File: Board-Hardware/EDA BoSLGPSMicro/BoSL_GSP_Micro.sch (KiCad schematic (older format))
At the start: 45 parts, among them CON1 Micro_SD_Card, CON2 BARREL_JACK, IC1 ATMEGA328-P, IC2 SIM7000, J7 USB_B_Micro, P2 CONN_01X04, P4 CONN_01X04, P7 CONN_01X04, SW1 SPST, U1 MCP1700T-3302E/TT, U3 MSQA6V1W5T2G, U4 74HC126, U5 FT232RL, Y1 8 MHz

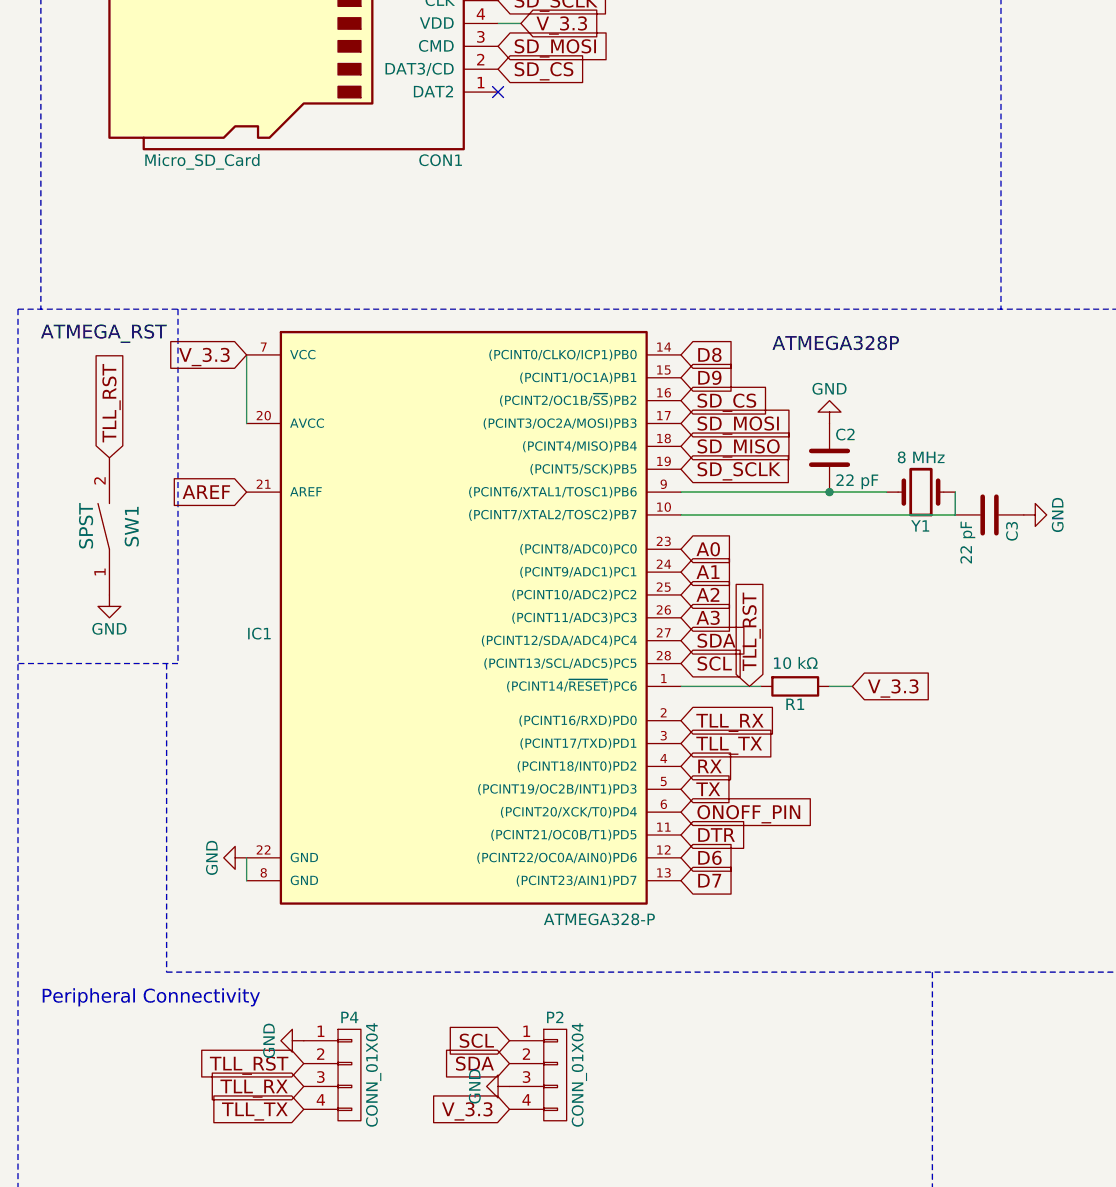
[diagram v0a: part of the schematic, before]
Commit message: layout progress of gps micro board
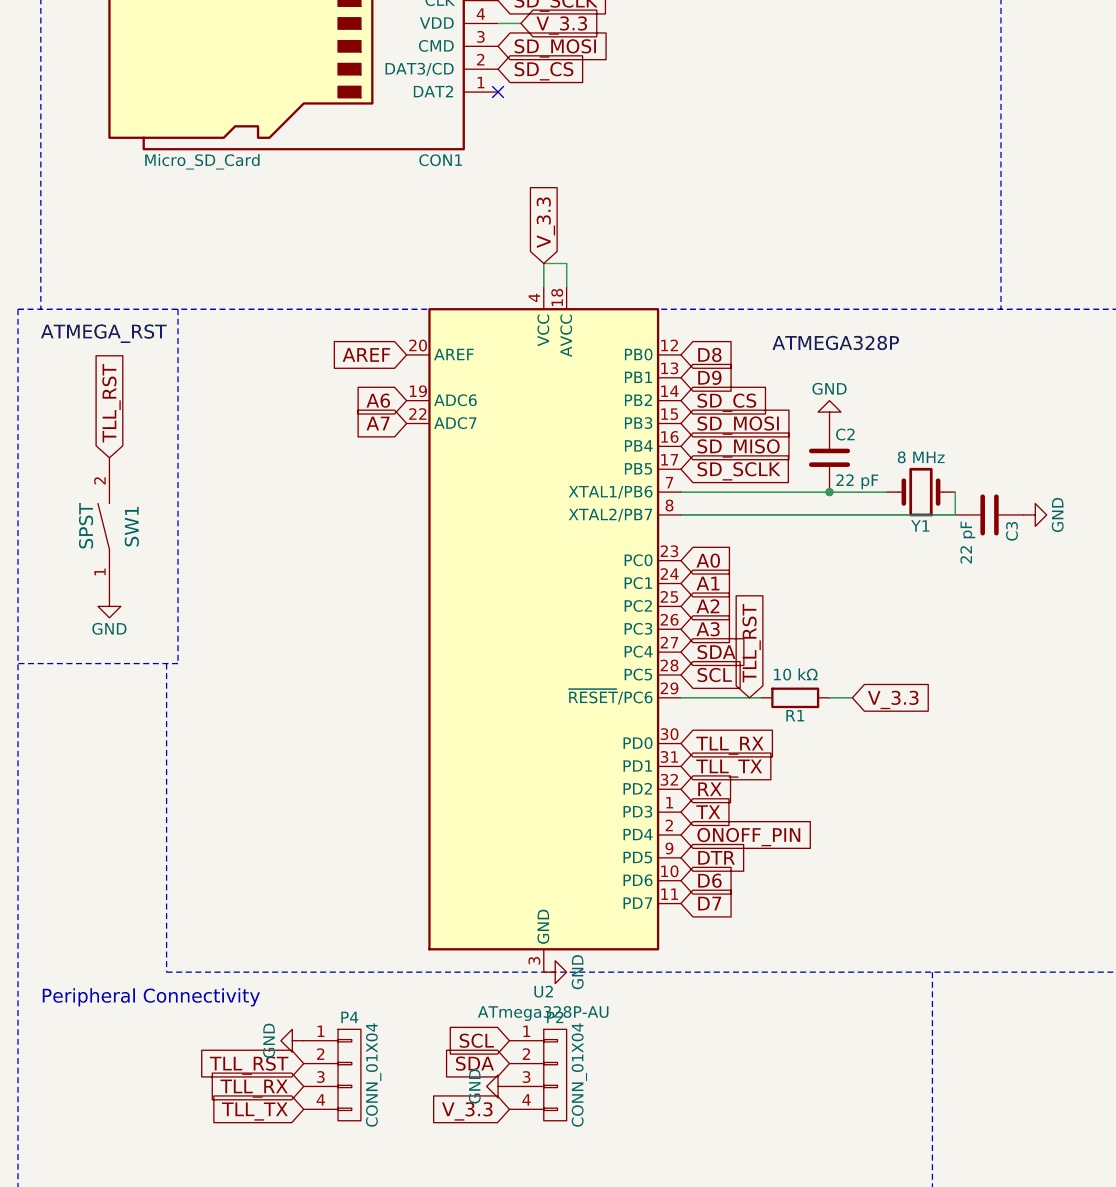
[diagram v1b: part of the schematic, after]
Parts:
- removed IC1: ATMEGA328-P, Housings_DIP:DIP-28_W7.62mm_Socket_LongPads, symbol SIM7000-rescue:ATMEGA328-P-SIM7000-rescue
- added U2: ATmega328P-AU, Housings_QFP:LQFP-32_7x7mm_Pitch0.8mm, symbol MCU_Microchip_ATmega:ATmega328P-AU
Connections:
- net A0: now also U2.23 (PC0)
- net A1: now also U2.24 (PC1)
- net A2: now also U2.25 (PC2)
- net A3: now also U2.26 (PC3)
- net AREF: now also U2.20 (AREF)
- net D6: now also U2.10 (PD6)
- net D7: now also U2.11 (PD7)
- net D8: now also U2.12 (PB0)
- net D9: now also U2.13 (PB1)
- net DTR: now also U2.9 (PD5)
- net GND: now also U2.21 (GND), U2.3 (GND), U2.5 (GND)
- net ONOFF_PIN: now also U2.2 (PD4)
- net RX: now also U2.32 (PD2)
- net SCL: now also U2.28 (PC5)
- net SDA: now also U2.27 (PC4)
- net SD_CS: now also U2.14 (PB2)
- net SD_MISO: now also U2.16 (PB4)
- net SD_MOSI: now also U2.15 (PB3)
- net SD_SCLK: now also U2.17 (PB5)
- net TLL_RST: now also U2.29 (~RESET~/PC6)
- net TLL_RX: now also U2.30 (PD0)
- net TLL_TX: now also U2.31 (PD1)
- net TX: now also U2.1 (PD3)
- net V_3.3: now also U2.18 (AVCC), U2.4 (VCC), U2.6 (VCC)
- net at C3.2, Y1.1: now also U2.8 (XTAL2/PB7)
- net at C2.2, Y1.2: now also U2.7 (XTAL1/PB6)
- new net A6: U2.19 (ADC6)
- new net A7: U2.22 (ADC7)
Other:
- moved on the sheet: R1
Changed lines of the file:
@@
 EESchema Schematic File Version 4
+LIBS:BoSL_GSP_Micro-cache
 EELAYER 29 0
 EELAYER END
@@
 NoConn ~ 7050 1500
 $Comp
-L SIM7000-rescue:ATMEGA328-P-SIM7000-rescue IC1
-U 1 1 5CE615FC
-P 2400 5050
-F 0 "IC1" H 1500 4900 50  0000 L BNN
-F 1 "ATMEGA328-P" H 2800 3650 50  0000 L BNN
-F 2 "Housings_DIP:DIP-28_W7.62mm_Socket_LongPads" H 2400 5050 50  0001 C CIN
-F 3 "" H 2400 5050 50  0000 C CNN
-	1    2400 5050
-	1    0    0    -1
-$EndComp
-$Comp
 L power:GND #PWR03
 U 1 1 5CE61B33
-P 1500 6150
-F 0 "#PWR03" H 1500 5900 50  0001 C CNN
-F 1 "GND" H 1500 6000 50  0000 C CNN
-F 2 "" H 1500 6150 50  0000 C CNN
-F 3 "" H 1500 6150 50  0000 C CNN
-	1    1500 6150
-	0    1    1    0
+P 2800 6650
+F 0 "#PWR03" H 2800 6400 50  0001 C CNN
+F 1 "GND" H 2800 6500 50  0000 C CNN
+F 2 "" H 2800 6650 50  0000 C CNN
+F 3 "" H 2800 6650 50  0000 C CNN
+	1    2800 6650
+	0    -1   -1   0
 $EndComp
 $Comp
 L Device:R R1
 U 1 1 5CE61DD3
-P 3900 5400
-F 0 "R1" V 3980 5400 50  0000 C CNN
-F 1 "10 kΩ" V 3800 5400 50  0000 C CNN
-F 2 "Resistors_SMD:R_0805_HandSoldering" V 3830 5400 50  0001 C CNN
-F 3 "" H 3900 5400 50  0000 C CNN
-	1    3900 5400
-	0    1    1    0
-$EndComp
-Text GLabel 3400 5950 2    60   Input ~ 0
+P 3900 5450
+F 0 "R1" V 3980 5450 50  0000 C CNN
+F 1 "10 kΩ" V 3800 5450 50  0000 C CNN
+F 2 "Resistors_SMD:R_0805_HandSoldering" V 3830 5450 50  0001 C CNN
+F 3 "" H 3900 5450 50  0000 C CNN
+	1    3900 5450
+	0    1    1    0
+$EndComp
+Text GLabel 3400 6050 2    60   Input ~ 0
 ONOFF_PIN
-Text GLabel 3700 5400 1    60   Input ~ 0
+Text GLabel 3700 5450 1    60   Input ~ 0
 TLL_RST
-Text GLabel 3400 5550 2    60   Input ~ 0
+Text GLabel 3400 5650 2    60   Input ~ 0
 TLL_RX
-Text GLabel 3400 5650 2    60   Input ~ 0
+Text GLabel 3400 5750 2    60   Input ~ 0
 TLL_TX
 $Comp
@@
 Text GLabel 1750 7050 0    60   Input ~ 0
 TLL_RST
-Text GLabel 3400 4800 2    60   Input ~ 0
+Text GLabel 3400 4850 2    60   Input ~ 0
 A0
-Text GLabel 3400 5200 2    60   Input ~ 0
+Text GLabel 3400 5250 2    60   Input ~ 0
 SDA
-Text GLabel 3400 5300 2    60   Input ~ 0
+Text GLabel 3400 5350 2    60   Input ~ 0
 SCL
-Text GLabel 3400 4900 2    60   Input ~ 0
+Text GLabel 3400 4950 2    60   Input ~ 0
 A1
-Text GLabel 3400 5000 2    60   Input ~ 0
+Text GLabel 3400 5050 2    60   Input ~ 0
 A2
-Text GLabel 3400 5100 2    60   Input ~ 0
+Text GLabel 3400 5150 2    60   Input ~ 0
 A3
 $Comp
@@
 Text GLabel 6550 2250 0    60   Input ~ 0
 DTR
-Text GLabel 3400 6050 2    60   Input ~ 0
+Text GLabel 3400 6150 2    60   Input ~ 0
 DTR
 $Comp
@@
 Text GLabel 3400 4450 2    60   Input ~ 0
 SD_SCLK
-Text GLabel 3400 5750 2    60   Input ~ 0
+Text GLabel 3400 5850 2    60   Input ~ 0
 RX
-Text GLabel 3400 5850 2    60   Input ~ 0
+Text GLabel 3400 5950 2    60   Input ~ 0
 TX
 Text GLabel 3400 4250 2    60   Input ~ 0
@@
 	1    0    0    -1
 $EndComp
-Text GLabel 3400 6250 2    60   Input ~ 0
+Text GLabel 3400 6350 2    60   Input ~ 0
 D7
 Text GLabel 3400 3950 2    60   Input ~ 0
 D8
-Text GLabel 1500 4550 0    60   Input ~ 0
+Text GLabel 2200 3950 0    60   Input ~ 0
 AREF
 $Comp
@@
 	7850 900  7850 1500
 Wire Wire Line
-	1500 6150 1500 6250
-Wire Wire Line
-	1500 4250 1500 3950
-Wire Wire Line
-	4150 5400 4050 5400
+	4150 5450 4050 5450
 Wire Wire Line
 	3400 4550 4050 4550
@@
 	0    1    1    0
 $EndComp
-Text GLabel 1500 3950 0    60   Input ~ 0
+Text GLabel 2800 3550 1    60   Input ~ 0
 V_3.3
 NoConn ~ 6550 3550
-Text GLabel 3400 6150 2    60   Input ~ 0
+Text GLabel 3400 6250 2    60   Input ~ 0
 D6
 Text GLabel 2650 7250 0    60   Input ~ 0
@@
 	14350 2400 14450 2400
 Wire Wire Line
-	3400 5400 3750 5400
+	3400 5450 3750 5450
 Wire Wire Line
 	8550 5000 9050 5000
@@
 Text Notes 9750 3800 0    60   ~ 0
 Mounting Holes\n
-Text GLabel 4150 5400 2    60   Input ~ 0
+Text GLabel 4150 5450 2    60   Input ~ 0
 V_3.3
 $Comp
@@
 	0    1    1    0
 $EndComp
+$Comp
+L MCU_Microchip_ATmega:ATmega328P-AU U2
+U 1 1 5DE0CED2
+P 2800 5150
+F 0 "U2" H 2800 3563 50  0000 C CNN
+F 1 "ATmega328P-AU" H 2800 3474 50  0000 C CNN
+F 2 "Housings_QFP:LQFP-32_7x7mm_Pitch0.8mm" H 2800 5150 50  0001 C CIN
+F 3 "http://ww1.microchip.com/downloads/en/DeviceDoc/ATmega328_P%20AVR%20MCU%20with%20picoPower%20Technology%20Data%20Sheet%2040001984A.pdf" H 2800 5150 50  0001 C CNN
+	1    2800 5150
+	1    0    0    -1
+$EndComp
+Wire Wire Line
+	2900 3650 2900 3550
+Wire Wire Line
+	2900 3550 2800 3550
+Wire Wire Line
+	2800 3650 2800 3550
+Text GLabel 2200 4150 0    60   Input ~ 0
+A6
+Text GLabel 2200 4250 0    60   Input ~ 0
+A7
 $EndSCHEMATC
